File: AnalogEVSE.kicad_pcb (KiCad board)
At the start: 2 copper layers, 102 x 85.7 mm, 80 parts, among them K1 Relay, P1 Pilot, P2 Rext, P3 230V, P4 Relay 1, P5 Status LEDs, P6 Power, P7 Relay 2, Q1 BC337-40, Q2 BC337-40, Q3 BC557, Q4 BC337-40, T1 12V/3VA, U1 LM2901, U2 LM7812, U3 LM7912, U4 LM2901

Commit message: RV2
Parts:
- C10: value 47n -> 150n
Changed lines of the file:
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@@
       (effects (font (size 1.016 1.016) (thickness 0.2032)))
     )
-    (fp_text value 47n (at 0 0) (layer F.SilkS) hide
+    (fp_text value 150n (at 0 0) (layer F.SilkS) hide
       (effects (font (size 1.016 1.016) (thickness 0.2032)))
     )

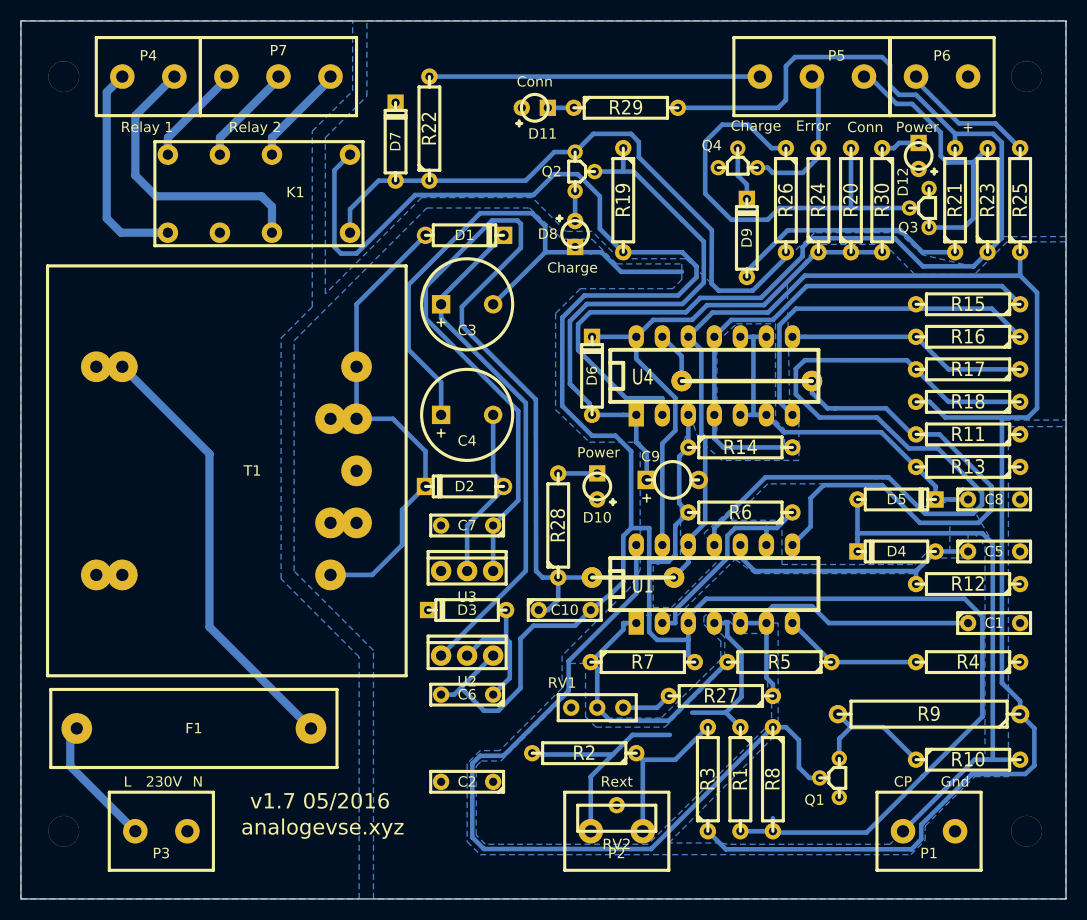
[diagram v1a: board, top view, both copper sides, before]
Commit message: Aetzwerk
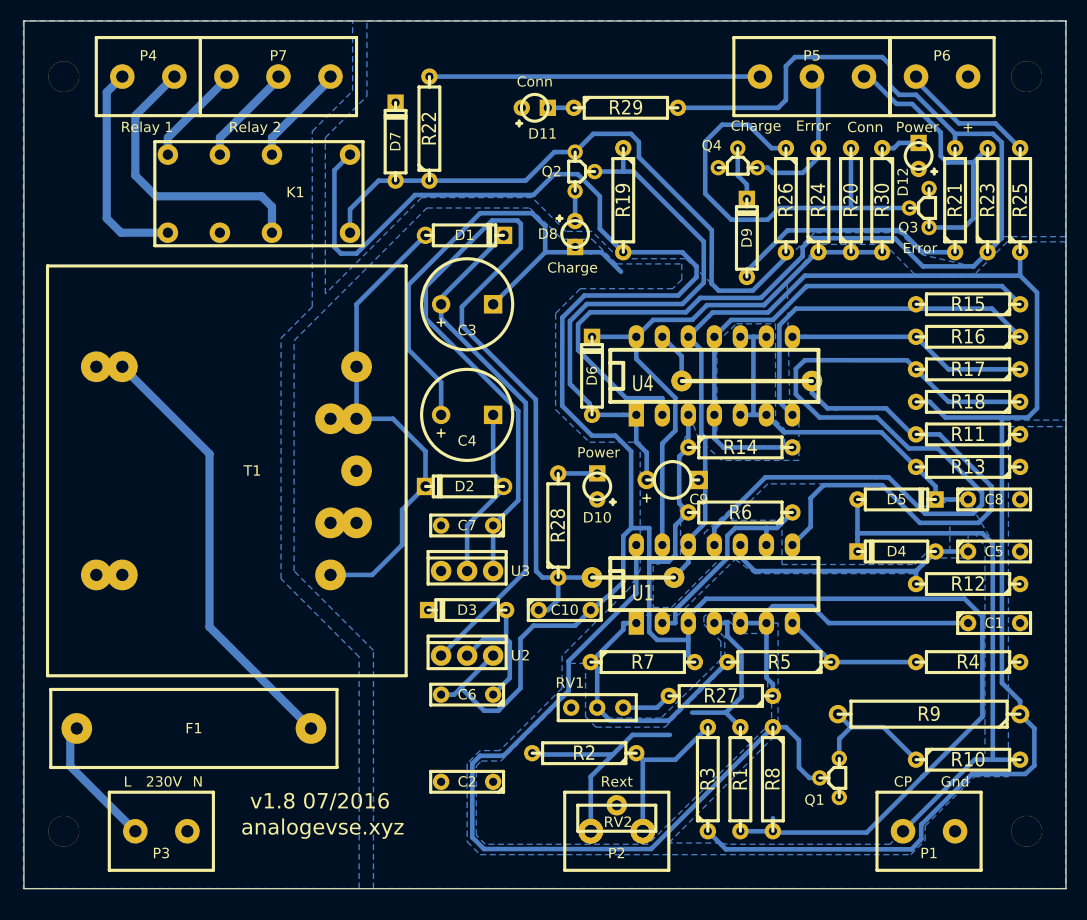
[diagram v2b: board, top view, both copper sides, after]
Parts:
- C3, C4: footprint mylib:C3 -> mylib:C5
- C9: footprint mylib:C4 -> mylib:C6
- RV2: footprint mylib:Trimpot2 -> mylib:Trimpot3
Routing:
- net GND: track 54.6 -> 48.7 mm
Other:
- board size 102 x 85.7 mm -> 101.7 x 84.7 mm
- board text added: "v1.8 07/2016"
- board text removed: "v1.7 05/2016"

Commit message: Addition of C11
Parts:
- R14: value 3k3 -> 4k7
- R15: value 2k7 -> 3k3
- R16: value 2k2 -> 5k6
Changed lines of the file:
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@@
       (effects (font (size 1.397 1.27) (thickness 0.2032)))
     )
-    (fp_text value 3k3 (at 0 0) (layer F.SilkS) hide
+    (fp_text value 4k7 (at 0 0) (layer F.SilkS) hide
       (effects (font (size 1.397 1.27) (thickness 0.2032)))
     )
@@
       (effects (font (size 1.397 1.27) (thickness 0.2032)))
     )
-    (fp_text value 2k7 (at 0 0 180) (layer F.SilkS) hide
+    (fp_text value 3k3 (at 0 0 180) (layer F.SilkS) hide
       (effects (font (size 1.397 1.27) (thickness 0.2032)))
     )
@@
       (effects (font (size 1.397 1.27) (thickness 0.2032)))
     )
-    (fp_text value 2k2 (at 0 0 180) (layer F.SilkS) hide
+    (fp_text value 5k6 (at 0 0 180) (layer F.SilkS) hide
       (effects (font (size 1.397 1.27) (thickness 0.2032)))
     )
